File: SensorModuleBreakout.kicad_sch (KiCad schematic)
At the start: 34 parts, among them J1 Conn_ST_STDC14, J2 Conn_01x10, J3 Conn_01x15, J4 Conn_01x03, J5 Conn_01x04, U1 STM32U031C8Tx, U2 SHT4x, U3 STC31-C-R3, U4 LPS22DF

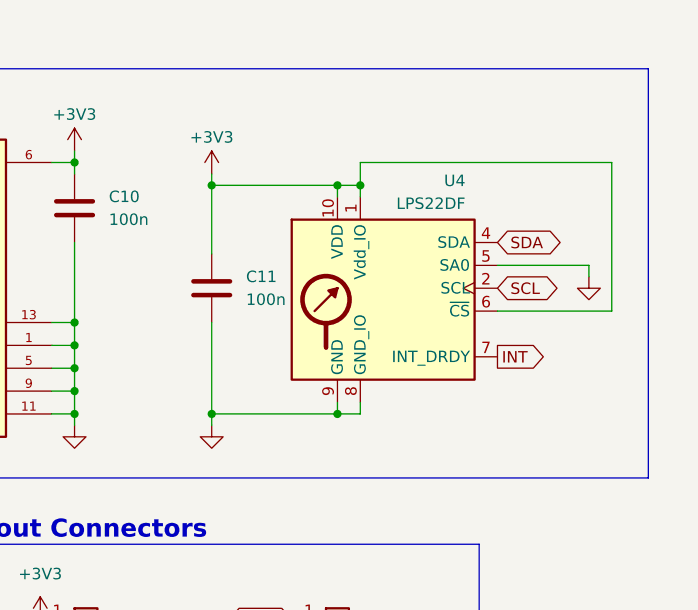
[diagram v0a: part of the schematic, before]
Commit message: update
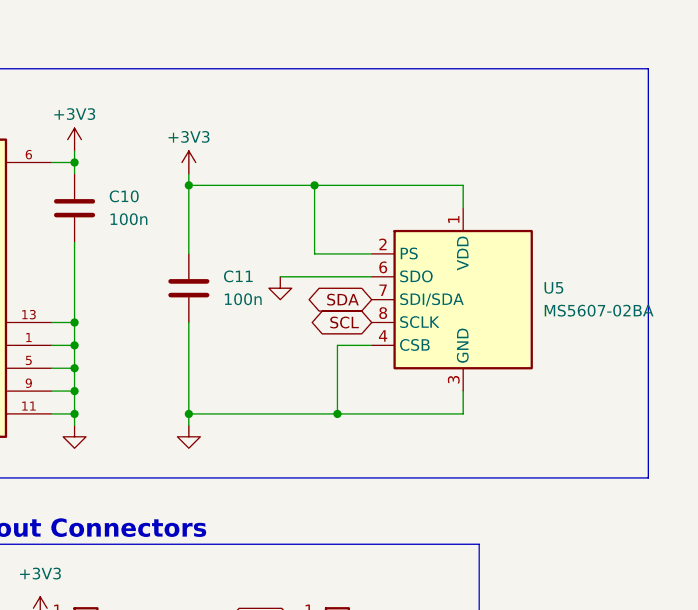
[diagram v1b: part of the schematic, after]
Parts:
- removed U4: LPS22DF, Package_LGA:ST_HLGA-10_2x2mm_P0.5mm_LayoutBorder3x2y, symbol Sensor_Pressure:LPS22DF
- added U5: MS5607-02BA, Package_LGA:LGA-8_3x5mm_P1.25mm, symbol Sensor_Pressure:MS5607-02BA
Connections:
- net +3V3: now also U5.1 (VDD), U5.2 (PS)
- net GND: now also U5.3 (GND), U5.4 (CSB), U5.5 (CSB), U5.6 (SDO)
- net SCL: now also U5.8 (SCLK)
- net SDA: now also U5.7 (SDI/SDA)
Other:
- moved on the sheet: C11
